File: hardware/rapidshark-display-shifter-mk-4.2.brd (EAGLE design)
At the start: 20.3 x 20.3 mm, 12 parts, among them U1 ADAFRUIT_FEATHER_SHIELDSMALLH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, U2 SPARKFUN_MICROVIEWSMALLHOLES

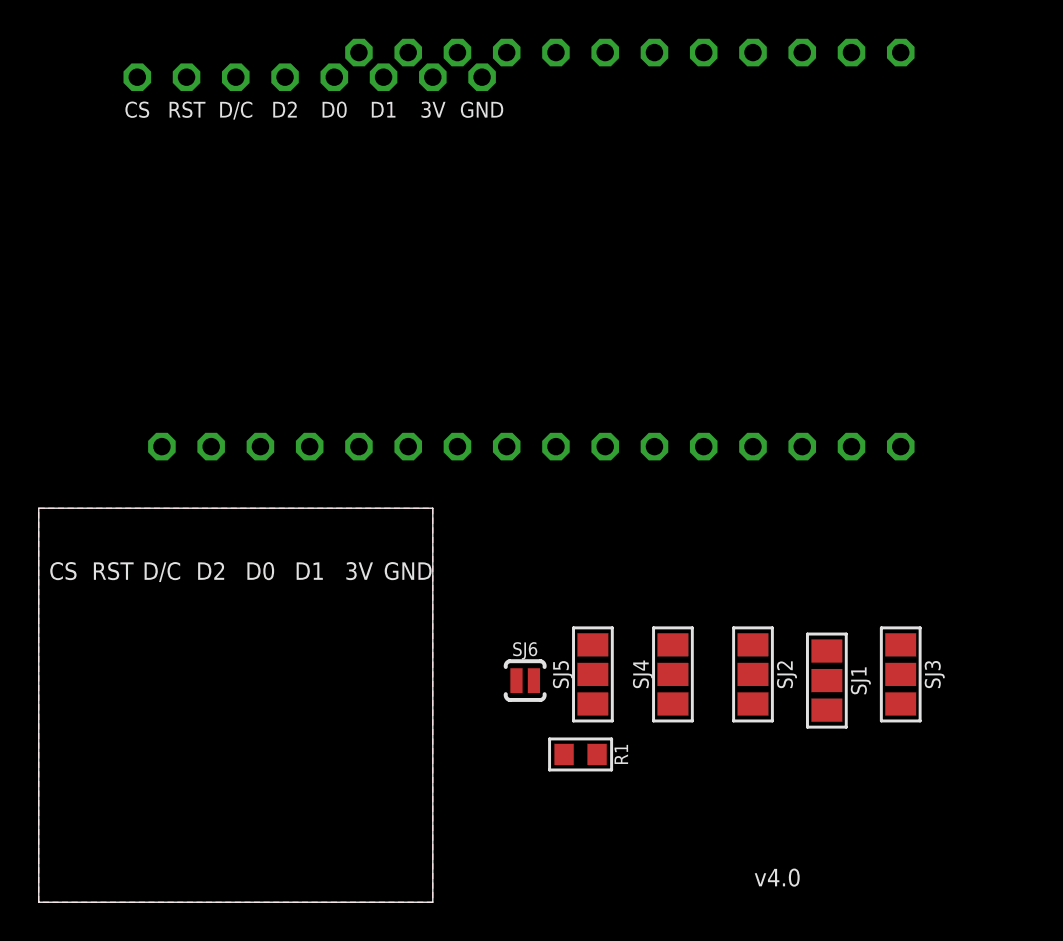
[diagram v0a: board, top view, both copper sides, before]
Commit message: adding these to commit to log before shifting to another repo
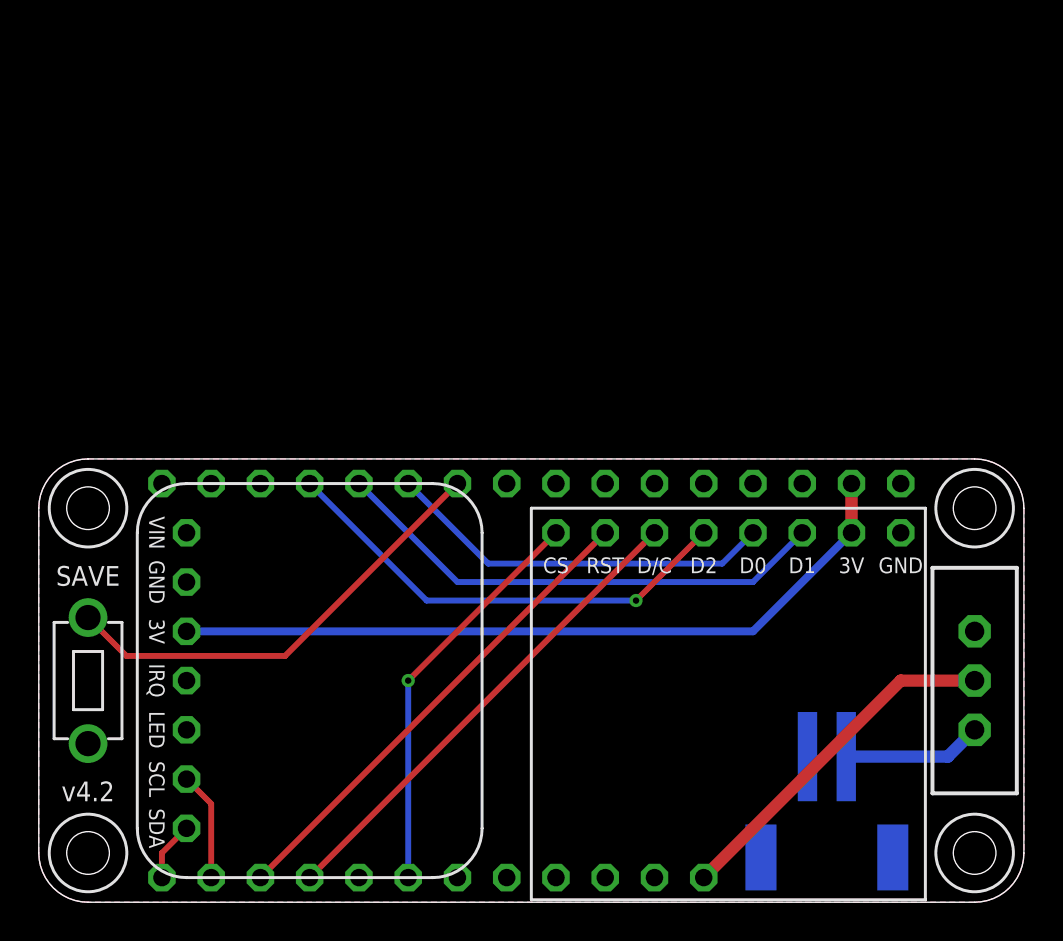
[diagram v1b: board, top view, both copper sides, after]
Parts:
- removed R1: 10K, a_parts:R0603
- removed SJ1, SJ2, SJ3, SJ4: I2C SPI, a_parts:PAD-JUMPER-3-NO_YES_SILK_FULL_BOX
- removed SJ5: 3C 3D, a_parts:PAD-JUMPER-3-NO_YES_SILK_FULL_BOX
- removed SJ6: JUMPER-PAD-2-NOYES_SILK, a_parts:PAD-JUMPER-2-NO_YES_SILK
- added BATT: M02JST-2MM-SMT, a_parts:JST-2-SMD
- added BUTT: SPST-NO-TACT3MM-PTH-SMALL-PADS, a_parts:DTS-3-SMALL-PADS
- added POWER: SWITCH-SPDTPTH-VERT-2.54MM, a_parts:SWITCH-SPDT
- added U3: ADAFRUIT-SI1145-BREAKOUTSMALLHOLES, a_parts:ADAFRUIT-SI1145-BREAKOUT-LESSSILK-SMALLHOLES
- moved U$3 37.2 mm to (2.54, 17.1)
- moved U2 31.9 mm to (35.6, 10.2)
- moved U1 22.2 mm to (25.4, 11.4), turned to 180 degrees
- moved U$1 18.7 mm to (25.4, 11.4)
- turned FRAME1 to 90 degrees
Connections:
- removed net D/C: U2.D/C
- removed net MISO: SJ3.3, U1.MISO
- removed net MOSI: SJ1.3, U1.MOSI
- removed net N$2: SJ4.1, SJ5.2
- removed net SCK: SJ2.3, U1.SCK
- removed net SHIELD_CS: SJ6.2, U1.10
- removed net SHIELD_D/C: SJ4.3, U1.6
- new net BUTT: BUTT.1, U1.A5
- new net DATA/CMD: U1.6, U2.D/C
- new net VBATT+: POWER.2, U1.BAT
- net 3.3V: now also U3.3V3_OUT; no longer R1.2
- net D0: now also U1.SCK; no longer SJ2.2
- net D1: now also U1.MOSI
- net D2: now also U1.MISO
- net DISP_CS: now also U1.10; no longer SJ6.1
- net GND: now also BATT.1, BUTT.2, U3.GND; no longer SJ5.3
- net N$1: now also BATT.2, POWER.1; no longer R1.1, SJ5.1
- net SCL: now also U3.SCL; no longer SJ2.1
- net SDA: now also U3.SDA; no longer SJ1.1
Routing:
- net 3.3V: track 0.00 -> 38.9 mm
- net D1: track 0.00 -> 26.0 mm
- net DISP_RST: track 0.00 -> 25.1 mm
- net DATA/CMD: track 0.00 -> 25.1 mm
- net D2: track 0.00 -> 24.3 mm, vias 0 -> 1
- net BUTT: track 0.00 -> 23.6 mm
- net DISP_CS: track 0.00 -> 20.9 mm, vias 0 -> 1
- net D0: track 0.00 -> 20.1 mm
- net VBATT+: track 0.00 -> 18.2 mm
- net N$1: track 0.00 -> 7.19 mm
- net SCL: track 0.00 -> 5.61 mm
- net SDA: track 0.00 -> 3.07 mm
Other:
- board size 20.3 x 20.3 mm -> 50.8 x 22.9 mm
- board text added: "SAVE"
- board text added: "UV Dosimeter Featherwing"
- board text removed: "3V"
- board text removed: "CS"
- board text removed: "D/C"
- board text removed: "D0"
- board text removed: "D1"
- board text removed: "D2"
- board text removed: "GND"
- board text removed: "RST"
